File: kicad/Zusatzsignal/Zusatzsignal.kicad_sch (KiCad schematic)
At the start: 3 parts, among them J1 VCC, J2 Zs

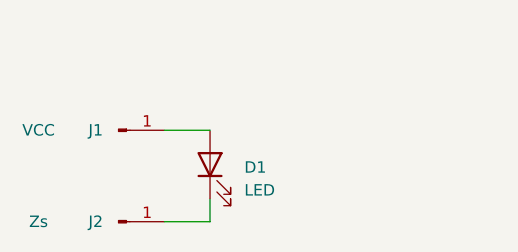
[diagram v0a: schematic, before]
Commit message: Add CC-BY-SA 4.0 license
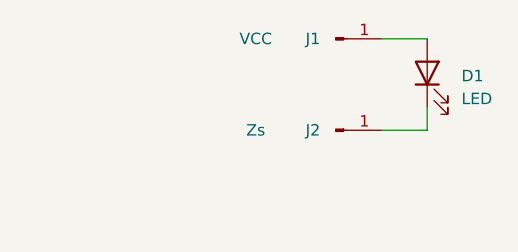
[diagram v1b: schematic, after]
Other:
- title: (none) -> KS-Zusatzsignal
- moved on the sheet: D1, J1, J2
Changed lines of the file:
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@@
-(kicad_sch (version 20211123) (generator eeschema)
-  (paper "A4")
-  (wire (pts (xy 81.28 76.2) (xy 86.36 76.2))
-    (stroke (width 0) (type default) (color 0 0 0 0))
+(kicad_sch (version 20230121) (generator eeschema)
+  (paper "A5")
+  (title_block
+    (title "KS-Zusatzsignal")
+    (date "2023-12-17")
+    (rev "1.0")
   )
-  (wire (pts (xy 86.36 76.2) (xy 86.36 73.66))
-    (stroke (width 0) (type default) (color 0 0 0 0))
+  (wire (pts (xy 105.41 66.04) (xy 110.49 66.04))
+    (stroke (width 0) (type default))
   )
-  (wire (pts (xy 81.28 66.04) (xy 86.36 66.04))
-    (stroke (width 0) (type default) (color 0 0 0 0))
+  (wire (pts (xy 110.49 66.04) (xy 110.49 63.5))
+    (stroke (width 0) (type default))
   )
-  (symbol (lib_id "Device:LED") (at 86.36 69.85 90) (unit 1)
-    (in_bom yes) (on_board yes) (fields_autoplaced)
-    (property "Reference" "D1" (id 0) (at 90.17 70.1674 90)
+  (wire (pts (xy 105.41 55.88) (xy 110.49 55.88))
+    (stroke (width 0) (type default))
+  )
+  (symbol (lib_id "Device:LED") (at 110.49 59.69 90) (unit 1)
+    (in_bom yes) (on_board yes) (dnp no) (fields_autoplaced)
+    (property "Reference" "D1" (at 114.3 60.0074 90)
       (effects (font (size 1.27 1.27)) (justify right))
     )
-    (property "Value" "LED" (id 1) (at 90.17 72.7074 90)
+    (property "Value" "LED" (at 114.3 62.5474 90)
       (effects (font (size 1.27 1.27)) (justify right))
     )
-    (property "Footprint" "LED_SMD:LED_0603_1608Metric" (id 2) (at 86.36 69.85 0)
+    (property "Footprint" "LED_SMD:LED_0603_1608Metric" (at 110.49 59.69 0)
       (effects (font (size 1.27 1.27)) hide)
     )
-    (property "Datasheet" "~" (id 3) (at 86.36 69.85 0)
+    (property "Datasheet" "~" (at 110.49 59.69 0)
       (effects (font (size 1.27 1.27)) hide)
     )
     (pin "1")
     (pin "2")
+    (instances
+      (project "Zusatzsignal"
+        (path "/e63e39d7-6ac0-4ffd-8aa3-1841a4541b55"
+          (reference "D1") (unit 1)
+        )
+      )
+    )
   )
-  (symbol (lib_id "Connector:Conn_01x01_Male") (at 76.2 76.2 0) (unit 1)
-    (in_bom yes) (on_board yes)
-    (property "Reference" "J2" (id 0) (at 73.66 76.2 0))
-    (property "Value" "Zs" (id 1) (at 67.31 76.2 0))
-    (property "Footprint" "Connector_Wire:SolderWirePad_1x01_SMD_1x2mm" (id 2) (at 76.2 76.2 0)
+  (symbol (lib_id "Connector:Conn_01x01_Male") (at 100.33 66.04 0) (unit 1)
+    (in_bom yes) (on_board yes) (dnp no)
+    (property "Reference" "J2" (at 97.79 66.04 0)
+      (effects (font (size 1.27 1.27)))
+    )
+    (property "Value" "Zs" (at 91.44 66.04 0)
+      (effects (font (size 1.27 1.27)))
+    )
+    (property "Footprint" "Connector_Wire:SolderWirePad_1x01_SMD_1x2mm" (at 100.33 66.04 0)
       (effects (font (size 1.27 1.27)) hide)
     )
-    (property "Datasheet" "~" (id 3) (at 76.2 76.2 0)
+    (property "Datasheet" "~" (at 100.33 66.04 0)
       (effects (font (size 1.27 1.27)) hide)
     )
     (pin "1")
+    (instances
+      (project "Zusatzsignal"
+        (path "/e63e39d7-6ac0-4ffd-8aa3-1841a4541b55"
+          (reference "J2") (unit 1)
+        )
+      )
+    )
   )
-  (symbol (lib_id "Connector:Conn_01x01_Male") (at 76.2 66.04 0) (unit 1)
-    (in_bom yes) (on_board yes)
-    (property "Reference" "J1" (id 0) (at 73.66 66.04 0))
-    (property "Value" "VCC" (id 1) (at 67.31 66.04 0))
-    (property "Footprint" "Connector_Wire:SolderWirePad_1x01_SMD_1x2mm" (id 2) (at 76.2 66.04 0)
+  (symbol (lib_id "Connector:Conn_01x01_Male") (at 100.33 55.88 0) (unit 1)
+    (in_bom yes) (on_board yes) (dnp no)
+    (property "Reference" "J1" (at 97.79 55.88 0)
+      (effects (font (size 1.27 1.27)))
+    )
+    (property "Value" "VCC" (at 91.44 55.88 0)
+      (effects (font (size 1.27 1.27)))
+    )
+    (property "Footprint" "Connector_Wire:SolderWirePad_1x01_SMD_1x2mm" (at 100.33 55.88 0)
       (effects (font (size 1.27 1.27)) hide)
     )
-    (property "Datasheet" "~" (id 3) (at 76.2 66.04 0)
+    (property "Datasheet" "~" (at 100.33 55.88 0)
       (effects (font (size 1.27 1.27)) hide)
     )
     (pin "1")
+    (instances
+      (project "Zusatzsignal"
+        (path "/e63e39d7-6ac0-4ffd-8aa3-1841a4541b55"
+          (reference "J1") (unit 1)
+        )
+      )
+    )
   )
   (sheet_instances
     (path "/" (page "1"))
   )
-  (symbol_instances
-    (path "/a3f3a018-6a6b-4914-95d4-b6f25692820f"
-      (reference "D1") (unit 1) (value "LED") (footprint "LED_SMD:LED_0603_1608Metric")
-    )
-    (path "/ebda1544-61d5-4166-a2e9-fde8904cbfc1"
-      (reference "J1") (unit 1) (value "VCC") (footprint "Connector_Wire:SolderWirePad_1x01_SMD_1x2mm")
-    )
-    (path "/e51e5768-e1af-448e-8d73-2a64bafc6c39"
-      (reference "J2") (unit 1) (value "Zs") (footprint "Connector_Wire:SolderWirePad_1x01_SMD_1x2mm")
-    )
-  )
 )
